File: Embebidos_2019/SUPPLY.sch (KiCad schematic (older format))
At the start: 25 parts, among them J4 Barrel_Jack_Switch, U3 ZLDO1117G33TA, U4 ZLDO1117G33TA, U5 TPS73201

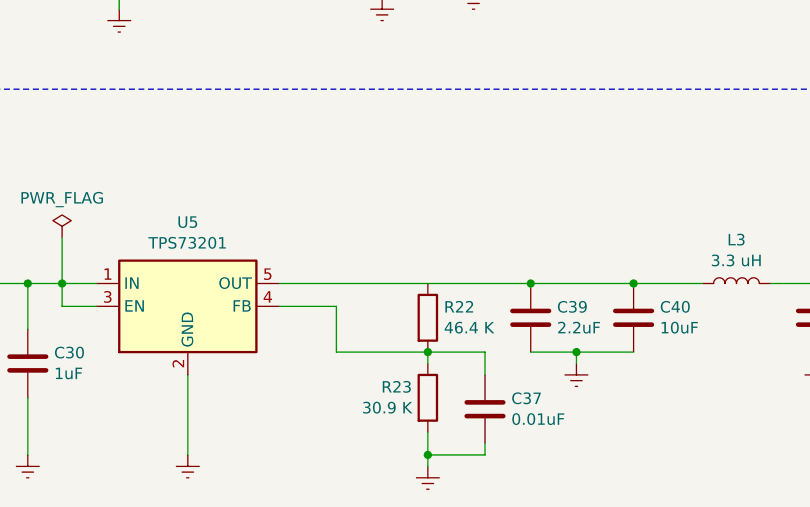
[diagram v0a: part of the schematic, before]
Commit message: Add files via upload
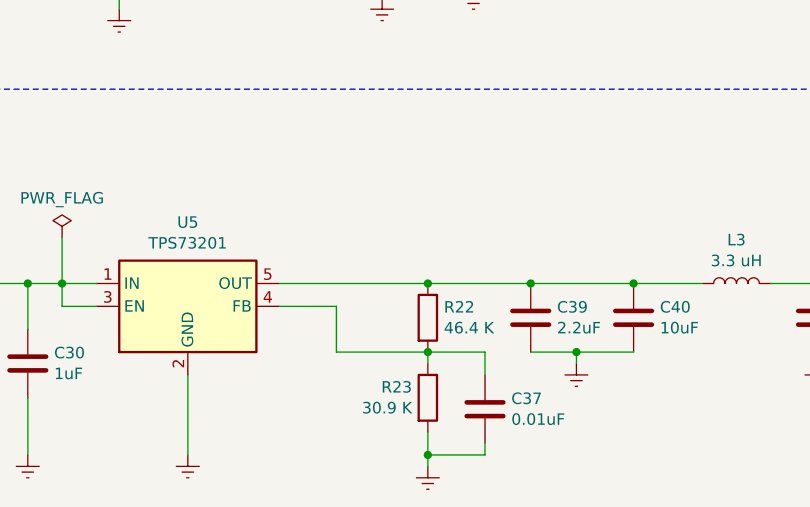
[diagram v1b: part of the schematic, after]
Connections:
- net at C39.1, C40.1, L3.1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: now also R22.1
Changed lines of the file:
@@
-EESchema Schematic File Version 4
+EESchema Schematic File Version 5
 LIBS:Embebidos_2019-cache
 EELAYER 29 0
@@
 	3400 8350 3400 8550
 Wire Wire Line
-	4350 8550 5450 8550
+	4350 8550 5000 8550
+Connection ~ 5000 8550
+Wire Wire Line
+	5000 8550 5450 8550
 $EndSCHEMATC

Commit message: ultima version
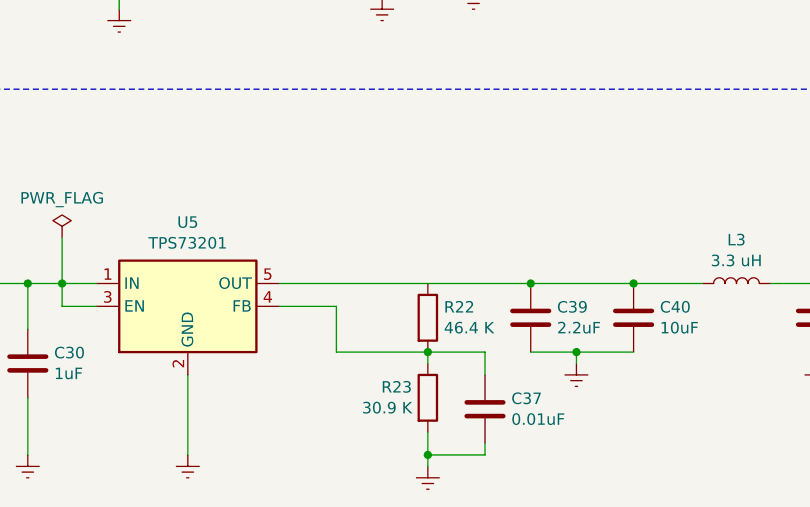
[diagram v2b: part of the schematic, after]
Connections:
- net at C39.1, C40.1, L3.1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: no longer R22.1
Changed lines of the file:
@@
-EESchema Schematic File Version 5
+EESchema Schematic File Version 4
 LIBS:Embebidos_2019-cache
 EELAYER 29 0
@@
 	3400 8350 3400 8550
 Wire Wire Line
-	4350 8550 5000 8550
-Connection ~ 5000 8550
-Wire Wire Line
-	5000 8550 5450 8550
+	4350 8550 5450 8550
 $EndSCHEMATC
